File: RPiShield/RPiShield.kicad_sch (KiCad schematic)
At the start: 6 parts, among them J2 BBOX, J4 Corridor1, J7 FC68148, J8 2223

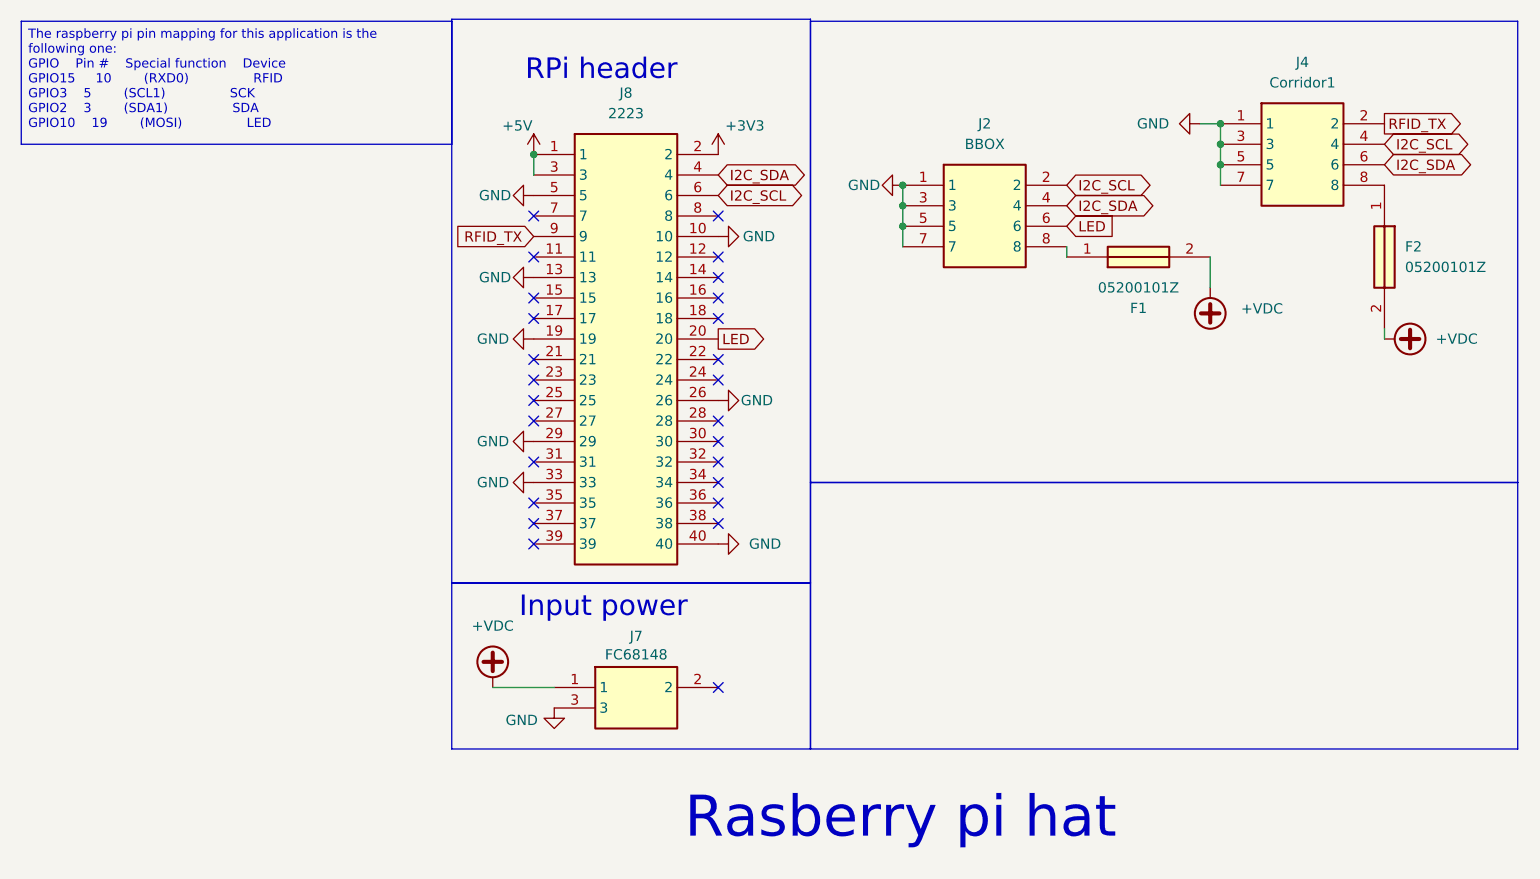
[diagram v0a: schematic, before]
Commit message: v1.0
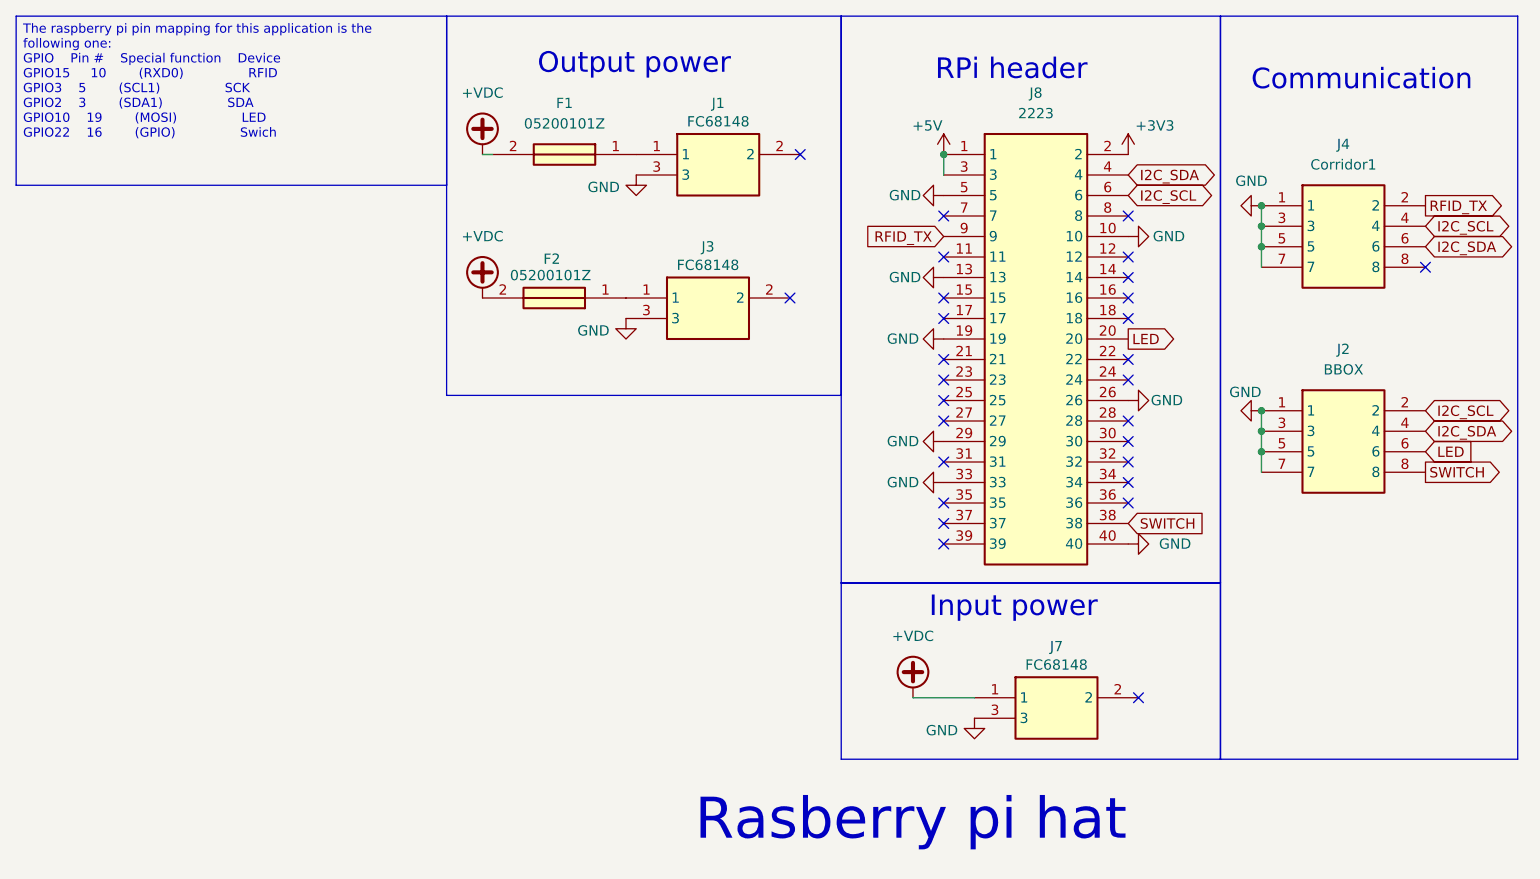
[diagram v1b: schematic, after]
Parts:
- added J1, J3: FC68148, FC68148:FC68148, symbol FC68148:FC68148
- F1, F2: footprint 05200101Z -> 05200101Z:05200101Z
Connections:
- net GND: now also J1.3, J3.3
- net at F1.1: now also J1.1; no longer J2.8
- net at F2.1: now also J3.1; no longer J4.8
- net SWITCH: now reaches J8.38
- net SWITCH: now also J2.8
- no-connect marks 26 -> 28
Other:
- note added: "Communication"
- note added: "Output power"
- moved on the sheet: F1, F2, J2, J4, J7, J8
